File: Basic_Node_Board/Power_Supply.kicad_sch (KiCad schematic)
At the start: 0 parts

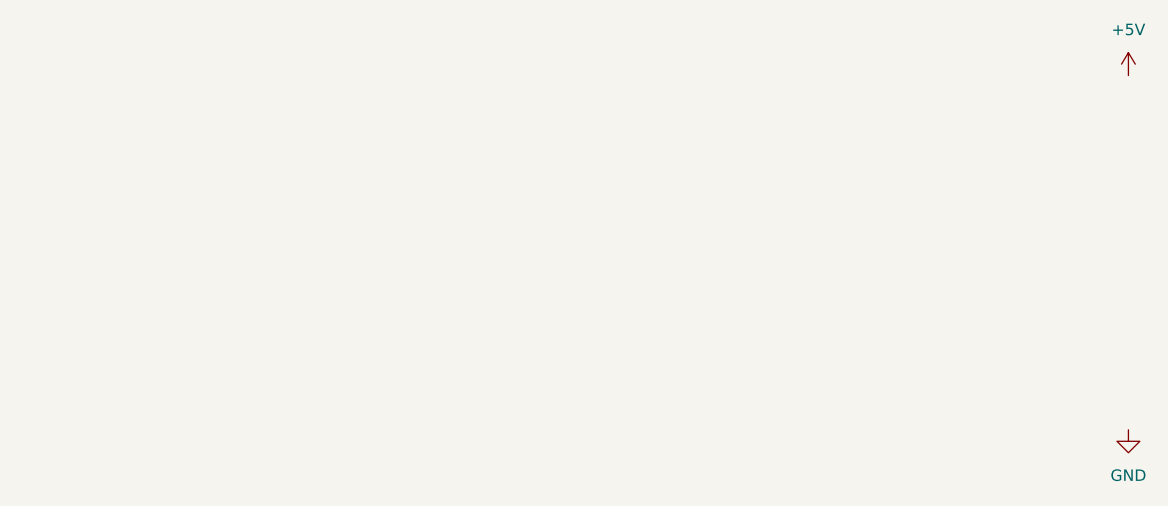
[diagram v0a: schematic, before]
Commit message: Initial PCB design for sensor board
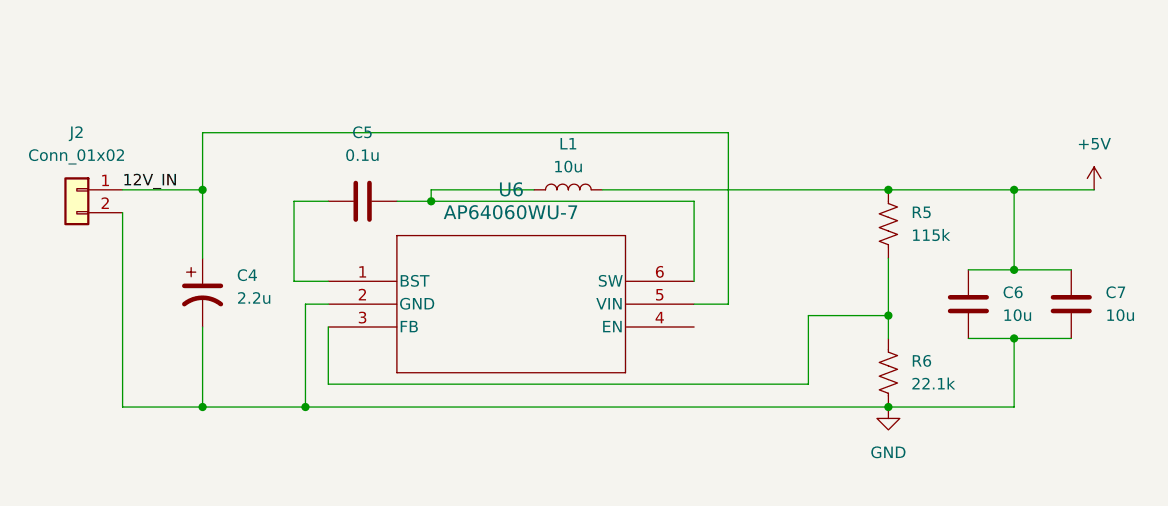
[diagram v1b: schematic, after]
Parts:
- added C4: 2.2u, Capacitor_SMD:CP_Elec_4x5.4, symbol PROVE:EEE-1VA2R2NR
- added C5: 0.1u, Capacitor_SMD:C_1206_3216Metric_Pad1.33x1.80mm_HandSolder, symbol PROVE:1206B104K500CT
- added C6, C7: 10u, Capacitor_SMD:C_1206_3216Metric_Pad1.33x1.80mm_HandSolder, symbol PROVE:CL31A106KPHNNNE
- added J2: Conn_01x02, TerminalBlock_TE-Connectivity:TerminalBlock_TE_282834-2_1x02_P2.54mm_Horizontal, symbol Connector_Generic:Conn_01x02
- added L1: 10u, PROVE:WE-LQS_5040, symbol PROVE:74404054100
- added R5: 115k, Resistor_SMD:R_1206_3216Metric_Pad1.30x1.75mm_HandSolder, symbol PROVE:RC1206FR-07115KL
- added R6: 22.1k, Resistor_SMD:R_1206_3216Metric_Pad1.30x1.75mm_HandSolder, symbol PROVE:RNCP1206FTD22K1
- added U6: AP64060WU-7, Package_TO_SOT_SMD:TSOT-23-6, symbol PROVE:AP64060WU-7
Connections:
- net +5V: now also C6.1, C7.1, L1.2, R5.1
- net GND: now also C4.2, C6.2, C7.2, J2.2 (Pin_2), R6.2, U6.2 (GND)
- new net: R5.2, R6.1, U6.3 (FB)
- new net: C5.2, L1.1, U6.6 (SW)
- new net: C5.1, U6.1 (BST)
- new net 12V_IN: C4.1, J2.1 (Pin_1), U6.5 (VIN)
